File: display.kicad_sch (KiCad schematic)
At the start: 26 parts, among them J701 Socket_Molex_SlimStack_2x20_5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, J702 HDMI-A_WE_685119134923

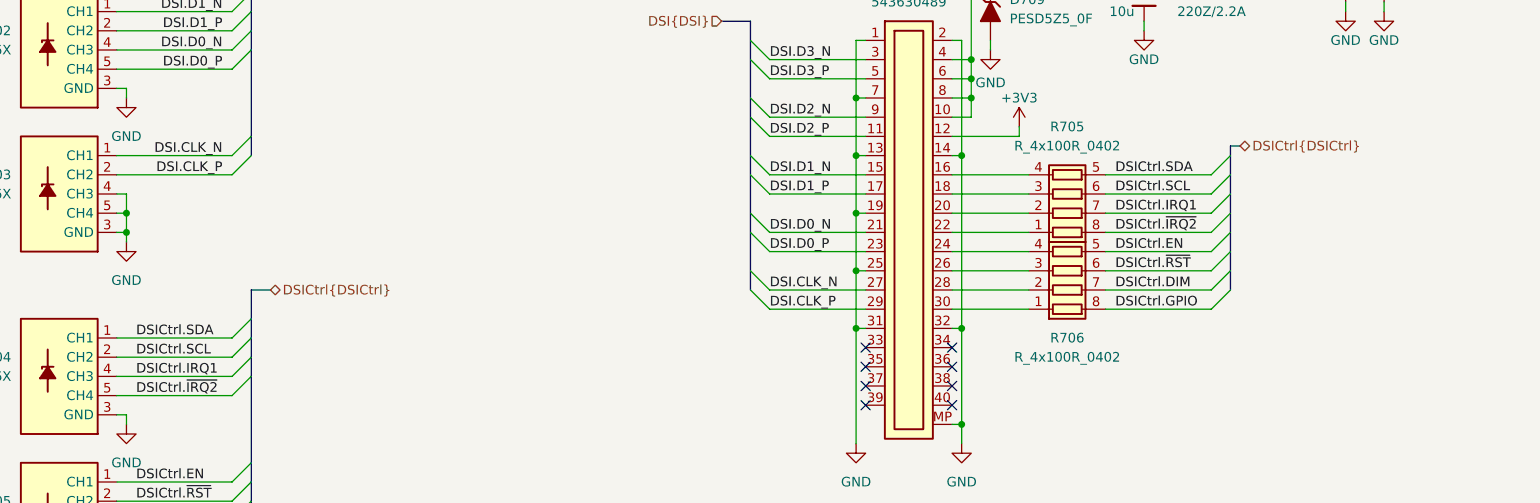
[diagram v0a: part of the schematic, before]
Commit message: [#55532] Sch: Optimize conections for easier routing
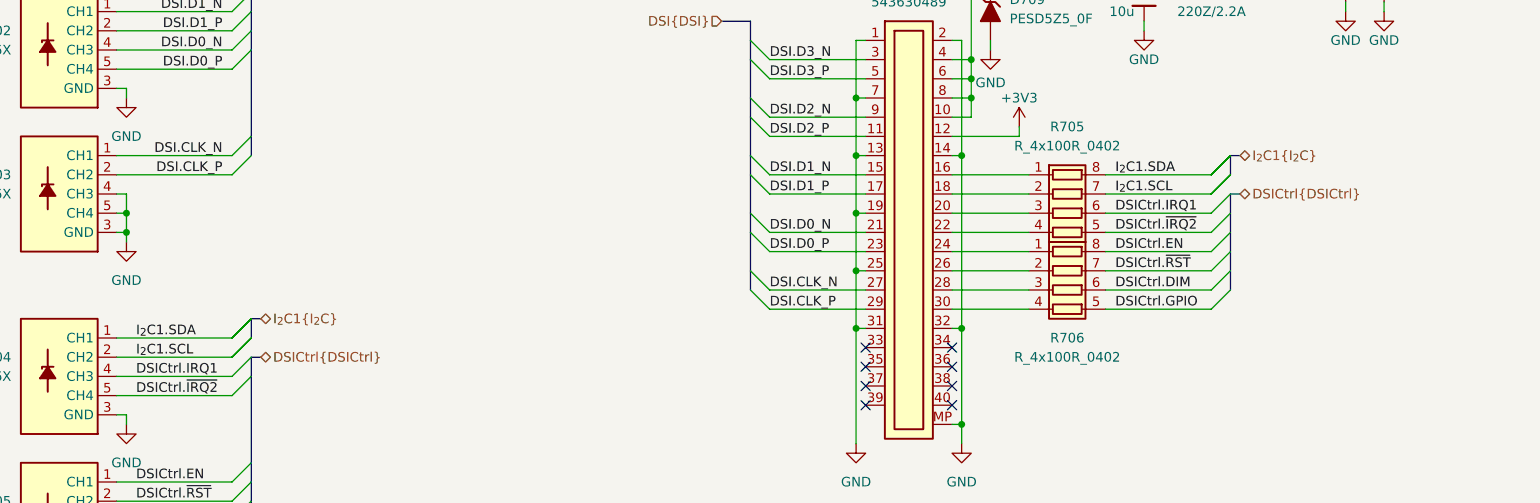
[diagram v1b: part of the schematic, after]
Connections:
- net DSICtrl.DIM: now also R706.6 (R3.2); no longer R706.7 (R2.2)
- net DSICtrl.EN: now also R706.8 (R1.2); no longer R706.5 (R4.2)
- net DSICtrl.GPIO: now also R706.5 (R4.2); no longer R706.8 (R1.2)
- net DSICtrl.IRQ1: now also R705.6 (R3.2); no longer R705.7 (R2.2)
- net DSICtrl.~{IRQ2}: now also R705.5 (R4.2); no longer R705.8 (R1.2)
- net DSICtrl.~{RST}: now also R706.7 (R2.2); no longer R706.6 (R3.2)
- net at J701.16: now also R705.1 (R1.1); no longer R705.4 (R4.1)
- net at J701.18: now also R705.2 (R2.1); no longer R705.3 (R3.1)
- net at J701.20: now also R705.3 (R3.1); no longer R705.2 (R2.1)
- net at J701.22: now also R705.4 (R4.1); no longer R705.1 (R1.1)
- net at J701.24: now also R706.1 (R1.1); no longer R706.4 (R4.1)
- net at J701.26: now also R706.2 (R2.1); no longer R706.3 (R3.1)
- net at J701.28: now also R706.3 (R3.1); no longer R706.2 (R2.1)
- net at J701.30: now also R706.4 (R4.1); no longer R706.1 (R1.1)
- net DSICtrl.SCL renamed I_{2}C1.SCL
- net I_{2}C1.SCL: now also R705.7 (R2.2); no longer R705.6 (R3.2)
- net DSICtrl.SDA renamed I_{2}C1.SDA
- net I_{2}C1.SDA: now also R705.8 (R1.2); no longer R705.5 (R4.2)
